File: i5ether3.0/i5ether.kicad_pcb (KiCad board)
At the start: 2 copper layers, 100 x 75 mm, 9 parts, among them J1 Conn_01x14, J2 7499011121A, J3 Conn_02x03_Counter_Clockwise, J4 Conn_01x04, P1 Conn_02x15_Counter_Clockwise, P2 Conn_02x15_Counter_Clockwise, P3 Conn_02x15_Counter_Clockwise, P4 Conn_02x15_Counter_Clockwise, P6 Conn_02x15_Counter_Clockwise

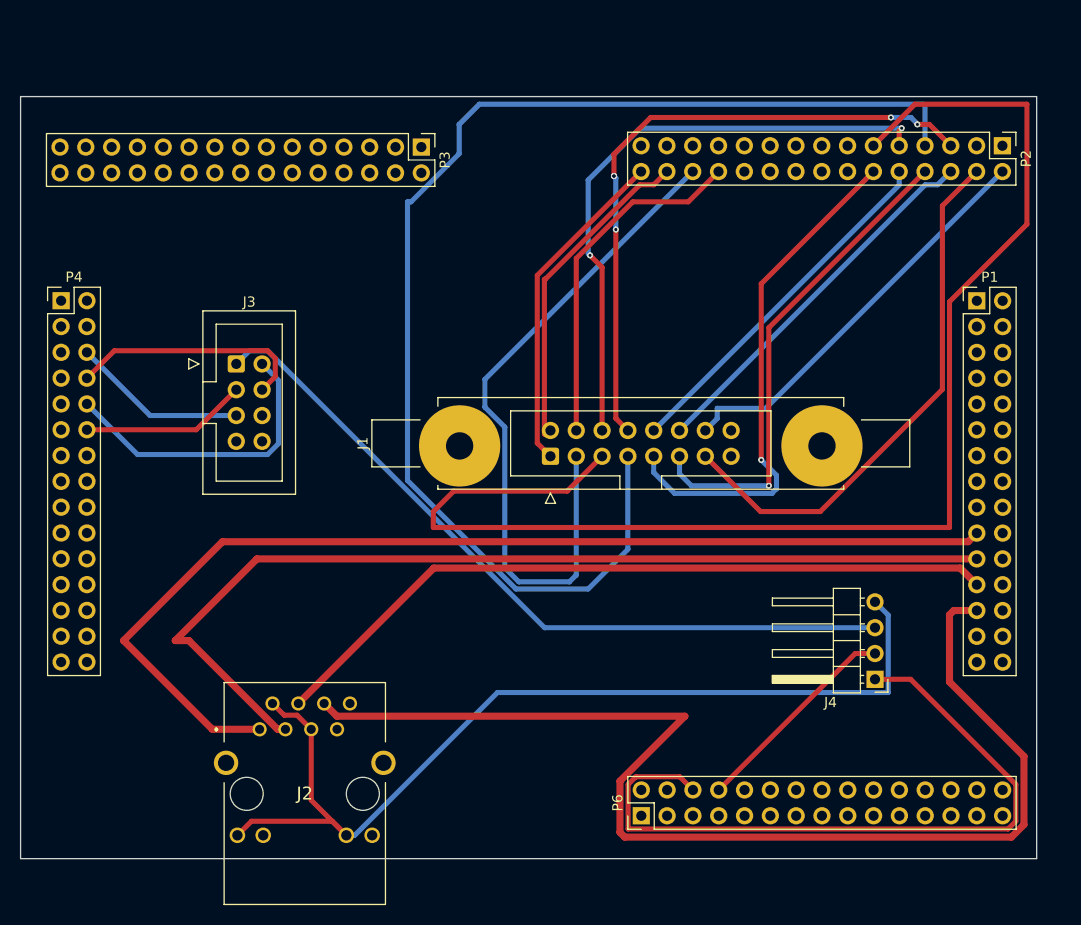
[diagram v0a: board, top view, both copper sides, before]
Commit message: PCB corecciones
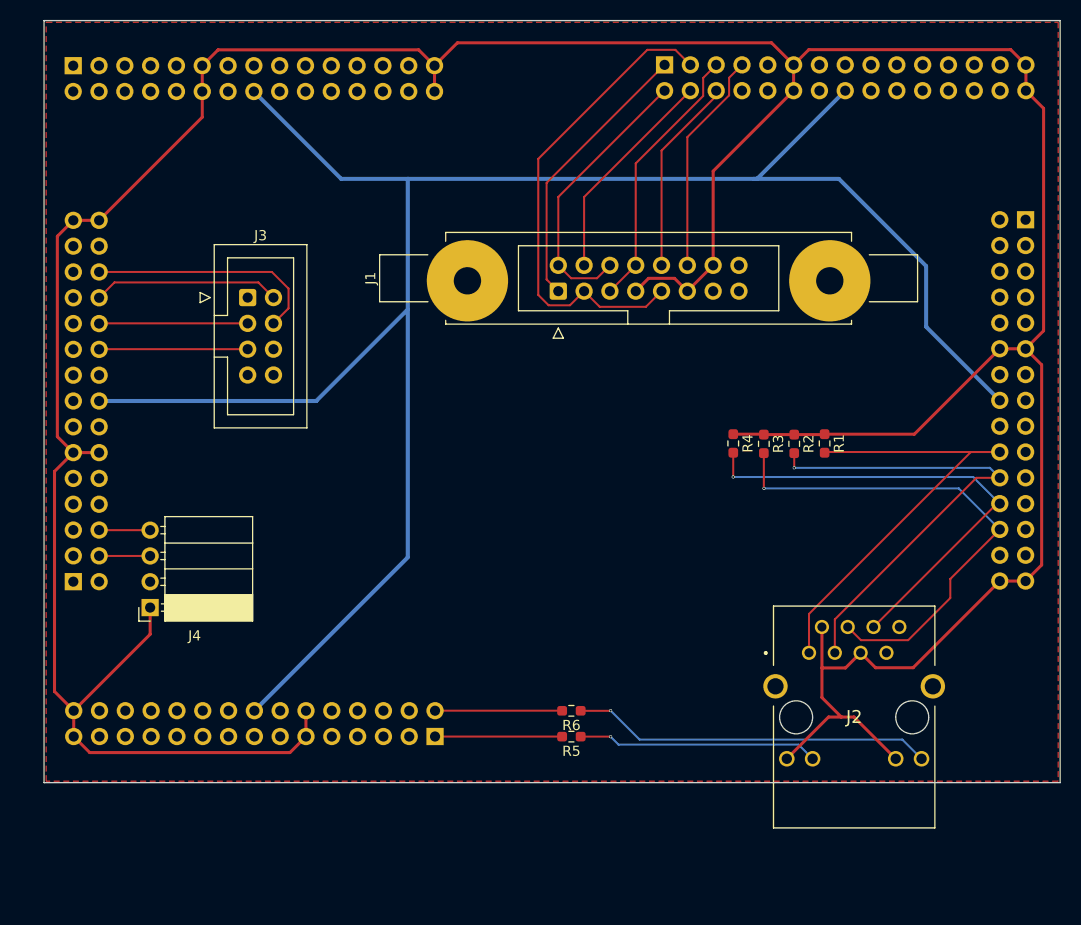
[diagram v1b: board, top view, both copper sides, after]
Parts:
- removed P6: Conn_02x15_Counter_Clockwise, Connector_PinHeader_2.54mm:PinHeader_2x15_P2.54mm_Vertical
- added P5: Conn_02x15_Counter_Clockwise, Connector_PinHeader_2.54mm:PinHeader_2x15_P2.54mm_Vertical, B.Cu at (134.8, 139.0)
- added R1: 50, Resistor_SMD:R_0603_1608Metric_Pad0.98x0.95mm_HandSolder, F.Cu at (173.1, 110.1)
- added R2: 50, Resistor_SMD:R_0603_1608Metric_Pad0.98x0.95mm_HandSolder, F.Cu at (170.1, 110.2)
- added R3: 50, Resistor_SMD:R_0603_1608Metric_Pad0.98x0.95mm_HandSolder, F.Cu at (167.2, 110.2)
- added R4: 50, Resistor_SMD:R_0603_1608Metric_Pad0.98x0.95mm_HandSolder, F.Cu at (164.1, 110.1)
- added R5: 330, Resistor_SMD:R_0603_1608Metric_Pad0.98x0.95mm_HandSolder, F.Cu at (148.2, 139.0)
- added R6: 330, Resistor_SMD:R_0603_1608Metric_Pad0.98x0.95mm_HandSolder, F.Cu at (148.2, 136.4)
- J4: footprint Connector_PinHeader_2.54mm:PinHeader_1x04_P2.54mm_Horizontal -> Connector_PinSocket_2.54mm:PinSocket_1x04_P2.54mm_Horizontal
- P1, P2, P3, P4: moved to B.Cu
- moved J4 71.7 mm to (106.8, 126.3)
- moved J2 54.6 mm to (176.0, 137.1)
- moved P3 35.2 mm to (99.2, 73.0)
- moved P2 34.2 mm to (157.4, 72.9)
- moved P4 27.7 mm to (99.2, 123.7)
- moved J1 16.3 mm to (146.9, 95.2)
- moved P1 9.31 mm to (192.9, 88.1), turned to 180 degrees
- moved J3 6.63 mm to (116.3, 95.8)
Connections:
- J1 pad 11: /screen_module/RESET -> +3.3V
- J1 pad 13: /screen_module/GND -> GND
- J1 pad 14: /screen_module/VCC -> +3.3V
- J1 pad 2: /screen_module/T_DO -> /screen_module/SDO(MISO)
- J1 pad 3: /screen_module/T_DIN -> /screen_module/SDI(MOSI)
- J1 pad 5: /screen_module/T_CLK -> /screen_module/SCK
- J1 pad 7: /screen_module/LED -> +3.3V
- J4 pad 1: /bluetooth_module/RX -> +3.3V
- J4 pad 2: /bluetooth_module/TX -> GND
- J4 pad 3: GND -> /bluetooth_module/TX
- J4 pad 4: +3.3V -> /bluetooth_module/RX
- P1 pad 10: unconnected-(P1-Pin_10-Pad10) -> GND
- P1 pad 11: unconnected-(P1-Pin_11-Pad11) -> +3.3V
- P1 pad 12: unconnected-(P1-Pin_12-Pad12) -> +3.3V
- P1 pad 15: unconnected-(P1-Pin_15-Pad15) -> GND
- P1 pad 16: unconnected-(P1-Pin_16-Pad16) -> +5V
- P1 pad 19: /ethernet_module/TD+ -> unconnected-(P1-Pin_19-Pad19)
- P1 pad 20: unconnected-(P1-Pin_20-Pad20) -> /ethernet_module/TD+
- P1 pad 21: /ethernet_module/TD- -> unconnected-(P1-Pin_21-Pad21)
- P1 pad 22: unconnected-(P1-Pin_22-Pad22) -> /ethernet_module/TD-
- P1 pad 23: /ethernet_module/RD+ -> unconnected-(P1-Pin_23-Pad23)
- P1 pad 24: unconnected-(P1-Pin_24-Pad24) -> /ethernet_module/RD-
- P1 pad 25: /ethernet_module/RD- -> unconnected-(P1-Pin_25-Pad25)
- P1 pad 26: unconnected-(P1-Pin_26-Pad26) -> /ethernet_module/RD+
- P1 pad 27: unconnected-(P1-Pin_27-Pad27) -> GND
- P1 pad 28: unconnected-(P1-Pin_28-Pad28) -> GND
- P1 pad 29: unconnected-(P1-Pin_29-Pad29) -> +3.3V
- P1 pad 30: unconnected-(P1-Pin_30-Pad30) -> +3.3V
- P1 pad 9: unconnected-(P1-Pin_9-Pad9) -> GND
- P2 pad 1: unconnected-(P2-Pin_1-Pad1) -> /screen_module/T_IRQ
- P2 pad 10: /screen_module/DC -> GND
- P2 pad 11: /screen_module/T_CLK -> +3.3V
- P2 pad 12: /screen_module/SDI(MOSI) -> +3.3V
- P2 pad 15: unconnected-(P2-Pin_15-Pad15) -> GND
- P2 pad 16: unconnected-(P2-Pin_16-Pad16) -> +5V
- P2 pad 2: /screen_module/VCC -> /screen_module/SDO(MISO)
- P2 pad 23: /ethernet_module/GLED- -> unconnected-(P2-Pin_23-Pad23)
- P2 pad 24: /screen_module/T_CS -> unconnected-(P2-Pin_24-Pad24)
- P2 pad 25: /ethernet_module/YLED- -> unconnected-(P2-Pin_25-Pad25)
- P2 pad 26: /screen_module/T_DIN -> unconnected-(P2-Pin_26-Pad26)
- P2 pad 27: unconnected-(P2-Pin_27-Pad27) -> GND
- P2 pad 28: /screen_module/T_DO -> GND
- P2 pad 29: unconnected-(P2-Pin_29-Pad29) -> +3.3V
- P2 pad 3: unconnected-(P2-Pin_3-Pad3) -> /screen_module/SDI(MOSI)
- P2 pad 30: /screen_module/T_IRQ -> +3.3V
- P2 pad 4: /screen_module/GND -> /screen_module/T_CS
- P2 pad 6: /screen_module/CS -> /screen_module/DC
- P2 pad 7: /screen_module/LED -> /screen_module/CS
- P2 pad 8: /screen_module/RESET -> unconnected-(P2-Pin_8-Pad8)
- P2 pad 9: /screen_module/SDO(MISO) -> GND
- P3 pad 10: unconnected-(P3-Pin_10-Pad10) -> GND
- P3 pad 11: unconnected-(P3-Pin_11-Pad11) -> +3.3V
- P3 pad 12: unconnected-(P3-Pin_12-Pad12) -> +3.3V
- P3 pad 15: unconnected-(P3-Pin_15-Pad15) -> GND
- P3 pad 16: unconnected-(P3-Pin_16-Pad16) -> +5V
- P3 pad 27: unconnected-(P3-Pin_27-Pad27) -> GND
- P3 pad 28: unconnected-(P3-Pin_28-Pad28) -> GND
- P3 pad 29: unconnected-(P3-Pin_29-Pad29) -> +3.3V
- P3 pad 30: unconnected-(P3-Pin_30-Pad30) -> +3.3V
- P3 pad 9: unconnected-(P3-Pin_9-Pad9) -> GND
- P4 pad 10: /SPI_module/RX -> GND
- P4 pad 11: unconnected-(P4-Pin_11-Pad11) -> +3.3V
- P4 pad 12: /SPI_module/CSn -> +3.3V
- P4 pad 15: unconnected-(P4-Pin_15-Pad15) -> GND
- P4 pad 16: unconnected-(P4-Pin_16-Pad16) -> +5V
- P4 pad 20: unconnected-(P4-Pin_20-Pad20) -> /SPI_module/TX
- P4 pad 22: unconnected-(P4-Pin_22-Pad22) -> /SPI_module/CSn
- P4 pad 24: unconnected-(P4-Pin_24-Pad24) -> /SPI_module/RX
- P4 pad 26: unconnected-(P4-Pin_26-Pad26) -> /SPI_module/SCK
- P4 pad 27: unconnected-(P4-Pin_27-Pad27) -> GND
- P4 pad 28: unconnected-(P4-Pin_28-Pad28) -> GND
- P4 pad 29: unconnected-(P4-Pin_29-Pad29) -> +3.3V
- P4 pad 30: unconnected-(P4-Pin_30-Pad30) -> +3.3V
- P4 pad 4: unconnected-(P4-Pin_4-Pad4) -> /bluetooth_module/TX
- P4 pad 6: /SPI_module/TX -> /bluetooth_module/RX
- P4 pad 8: /SPI_module/SCK -> unconnected-(P4-Pin_8-Pad8)
- P4 pad 9: unconnected-(P4-Pin_9-Pad9) -> GND
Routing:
- net +3.3V: track 97.2 -> 373.2 mm
- net +5V: track 0.00 -> 194.8 mm
- net /screen_module/T_CLK: track 132.9 -> 0.00 mm
- net /screen_module/LED: track 124.9 -> 0.00 mm
- net GND: track 74.7 -> 0.00 mm
- net /ethernet_module/RD-: track 118.0 -> 47.2 mm, vias 0 -> 1
- net /screen_module/T_DIN: track 67.9 -> 0.00 mm
- net /bluetooth_module/RX: track 71.9 -> 5.24 mm
- net /ethernet_module/TD+: track 105.4 -> 46.5 mm
- net /screen_module/GND: track 53.4 -> 0.00 mm
- net /ethernet_module/TD-: track 97.8 -> 47.4 mm, vias 0 -> 1
- net /screen_module/RESET: track 48.3 -> 0.00 mm, vias 1 -> 0
- net /screen_module/VCC: track 40.4 -> 0.00 mm
- net /screen_module/SCK: track 63.7 -> 26.6 mm, vias 5 -> 0
- net Net-(J2-Pad12): track 0.00 -> 35.5 mm, vias 0 -> 1
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- added copper zone on F.Cu, net GND
